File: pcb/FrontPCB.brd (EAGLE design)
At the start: 128.4 x 25.1 mm, 0 parts

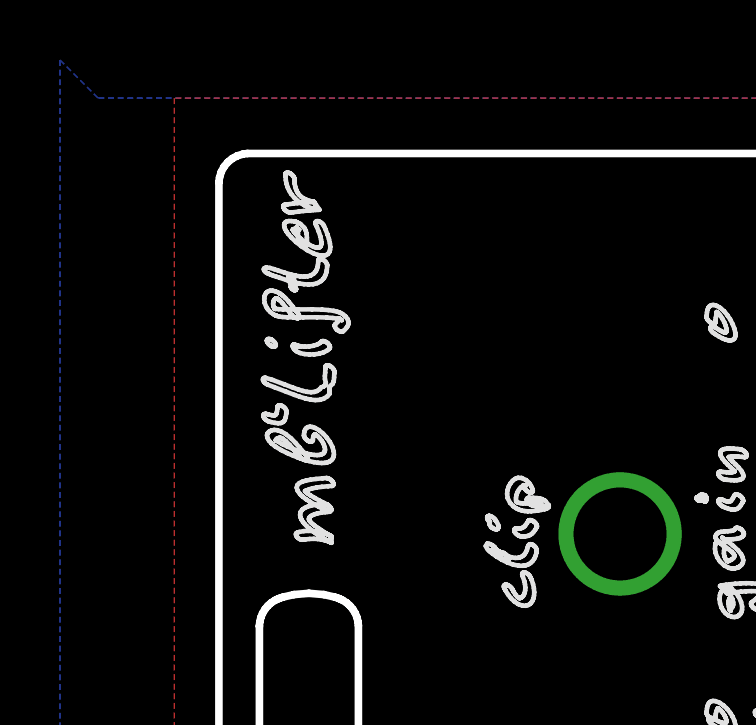
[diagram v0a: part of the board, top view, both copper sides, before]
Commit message: BigMac changes.
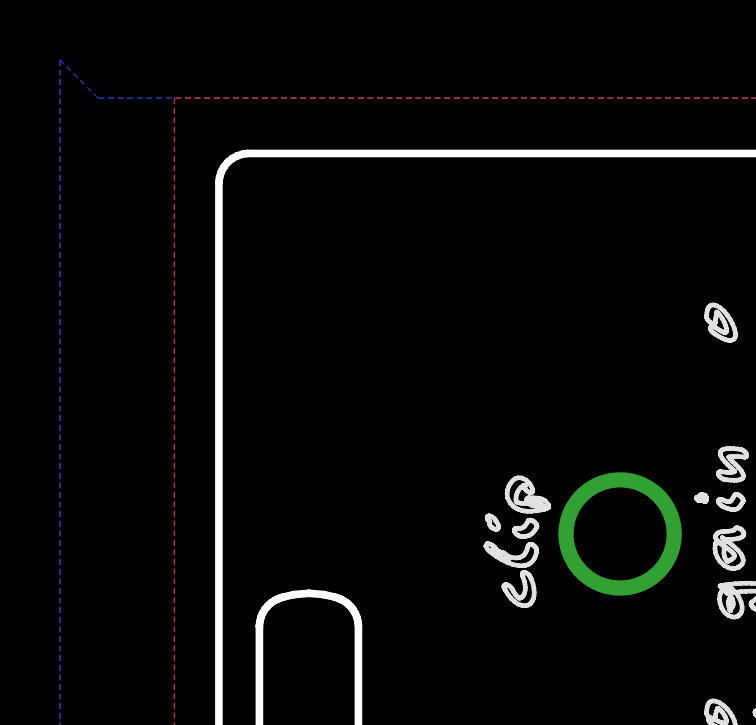
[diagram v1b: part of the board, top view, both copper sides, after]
